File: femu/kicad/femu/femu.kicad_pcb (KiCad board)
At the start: 6 copper layers, 13 x 9.4 mm, 11 parts, among them U1 ESP32-D2WD, U2 FT231XQ, U3 LDO, Y1 ECS-TXO-2016-33-400-TR

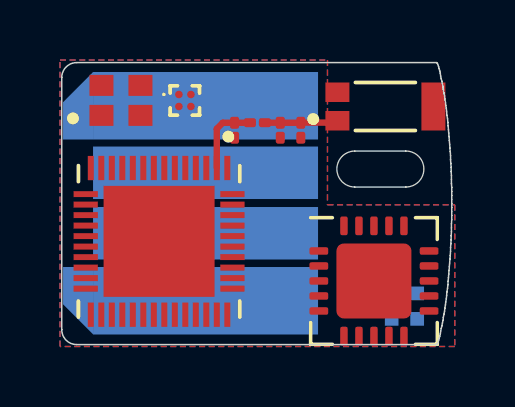
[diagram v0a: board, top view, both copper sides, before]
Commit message: KiCAD design updates
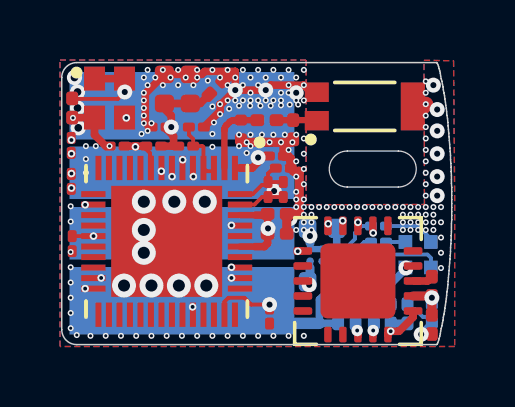
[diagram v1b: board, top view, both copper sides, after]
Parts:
- added C10: 2.2uF, Capacitor_SMD:C_0402_1005Metric, B.Cu at (135.7, 97.7)
- added C11: 2.2uF, Capacitor_SMD:C_0402_1005Metric, B.Cu at (135.7, 99.5)
- added C12: 0.1uF, Capacitor_SMD:C_0201_0603Metric, F.Cu at (127.4, 93.7)
- added C13: 10nF, Capacitor_SMD:C_01005_0402Metric, F.Cu at (134.4, 95.7)
- added C14: 0.22uF, Capacitor_SMD:C_01005_0402Metric, F.Cu at (130.3, 94.4)
- added C15: 2.2uF, Capacitor_SMD:C_0201_0603Metric, F.Cu at (134.2, 97.9)
- added C16: 100pF, Capacitor_SMD:C_0201_0603Metric, F.Cu at (134.2, 97.3)
- added C17: 0.22uF, Capacitor_SMD:C_01005_0402Metric, F.Cu at (127.4, 98.2)
- added C18: 22uF, Capacitor_SMD:C_0402_1005Metric, F.Cu at (130.5, 93.1)
- added C19: 3.3nF, Capacitor_SMD:C_01005_0402Metric, F.Cu at (133.9, 96.4)
- added C20: 270PF, Capacitor_SMD:C_01005_0402Metric, F.Cu at (127.4, 96.2)
- added C21: 0.22uF, Capacitor_SMD:C_01005_0402Metric, F.Cu at (134.0, 100.7)
- added C22: 22uF, Capacitor_SMD:C_0402_1005Metric, F.Cu at (131.3, 93.1)
- added C23: 2.2uF, Capacitor_SMD:C_0201_0603Metric, F.Cu at (132.2, 93.0)
- added C24: 0.22uF, Capacitor_SMD:C_01005_0402Metric, F.Cu at (134.2, 95.3)
- added C25: 0.22uF, Capacitor_SMD:C_01005_0402Metric, F.Cu at (128.9, 95.0)
- added C26: DNP, Capacitor_SMD:C_01005_0402Metric, F.Cu at (131.5, 94.4)
- added C4: 0.22uF, Capacitor_SMD:C_0201_0603Metric, F.Cu at (139.4, 99.7)
- added C5: 4.7uF, Capacitor_SMD:C_0201_0603Metric, F.Cu at (139.4, 100.9)
- added C6: 0.22uF, Capacitor_SMD:C_0201_0603Metric, B.Cu at (138.6, 100.6)
- added C7: 47pF, Capacitor_SMD:C_0201_0603Metric, B.Cu at (137.1, 99.5)
- added C8: 47pF, Capacitor_SMD:C_0201_0603Metric, B.Cu at (136.3, 100.6)
- added C9: 10nF, Capacitor_SMD:C_0201_0603Metric, B.Cu at (139.4, 100.6)
- added L2: L, Inductor_SMD:L_01005_0402Metric, F.Cu at (131.2, 95.0)
- added R1: 0, Resistor_SMD:R_0201_0603Metric, B.Cu at (138.0, 100.6)
- added R2: 27, Resistor_SMD:R_0201_0603Metric, B.Cu at (137.5, 100.6)
- added R3: 27, Resistor_SMD:R_0201_0603Metric, B.Cu at (136.9, 100.6)
- added R4: 270, Resistor_SMD:R_01005_0402Metric, B.Cu at (137.6, 98.2)
- added R5: 270, Resistor_SMD:R_01005_0402Metric, B.Cu at (137.6, 97.7)
- added R6: 270, Resistor_SMD:R_01005_0402Metric, B.Cu at (137.6, 98.8)
- added R7: 10K, Resistor_SMD:R_01005_0402Metric, F.Cu at (130.1, 95.0)
- added R8: 20K (5%), Resistor_SMD:R_01005_0402Metric, F.Cu at (134.4, 96.4)
- C1: value C_Small -> 270PF
- C2, C3: footprint Capacitor_SMD:C_01005_0402Metric -> Capacitor_SMD:C_0201_0603Metric
- L1: footprint Inductor_SMD:L_01005_0402Metric -> Inductor_SMD:L_0201_0603Metric
- U3: moved to B.Cu
- moved C1 7.67 mm to (127.4, 95.0), turned to 90 degrees
- moved U3 6.76 mm to (135.5, 98.6), turned to -90 degrees
- moved LED1 1.77 mm to (138.9, 98.6), turned to -90 degrees
- moved USB1 0.79 mm to (131.1, 96.9)
- moved ANT1 0.69 mm to (137.2, 93.7)
- moved U2 0.53 mm to (136.9, 99.5)
- moved C2 0.43 mm to (134.8, 94.4)
- moved Y1 0.39 mm to (128.7, 93.4), turned to -90 degrees
- moved C3 0.33 mm to (133.9, 94.1)
- moved U1 0.25 mm to (130.6, 98.2)
- moved L1 0.21 mm to (133.0, 94.4)
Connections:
- C1 pad 1: Net-(ANT1-PadFEED) -> Net-(C1-Pad1)
- C1 pad 2: GND -> Net-(C1-Pad2)
- LED1 pad 1: Net-(LED1-Pad1) -> +3V3
- U1 pad 1: Net-(U1-Pad1) -> +3V3
- U1 pad 16: Net-(U1-Pad16) -> /IO27_R
- U1 pad 19: Net-(U1-Pad19) -> +3V3
- U1 pad 23: Net-(U1-Pad23) -> /BOOT_DTR
- U1 pad 24: Net-(U1-Pad24) -> /IO4_G
- U1 pad 34: Net-(U1-Pad34) -> /IO5_B
- U1 pad 37: Net-(U1-Pad37) -> +3V3
- U1 pad 40: Net-(U1-Pad40) -> /UART-
- U1 pad 41: Net-(U1-Pad41) -> /UART+
- U1 pad 43: Net-(U1-Pad1) -> +3V3
- U1 pad 46: Net-(U1-Pad1) -> +3V3
- U1 pad 7: Net-(U1-Pad7) -> Net-(C1-Pad2)
- U1 pad 8: Net-(U1-Pad8) -> Net-(C1-Pad1)
- U1 pad 9: Net-(U1-Pad9) -> /EN_RTS
- U2 pad 1: Net-(U2-Pad1) -> /UART+
- U2 pad 10: Net-(U2-Pad10) -> Net-(C6-Pad1)
- U2 pad 11: Net-(U2-Pad11) -> Net-(C6-Pad1)
- U2 pad 12: Net-(U2-Pad12) -> +5V
- U2 pad 17: Net-(U2-Pad17) -> /UART-
- U2 pad 18: Net-(U2-Pad18) -> /BOOT_DTR
- U2 pad 19: Net-(U2-Pad19) -> /EN_RTS
- U2 pad 20: Net-(U2-Pad20) -> Net-(C6-Pad1)
- U2 pad 8: Net-(U2-Pad8) -> /USB+
- U2 pad 9: Net-(U2-Pad9) -> /USB-
- U3 pad A1: Net-(U3-PadA1) -> +5V
- U3 pad A2: Net-(U3-PadA2) -> +3V3
- U3 pad B1: Net-(U3-PadB1) -> +5V
- USB1 pad 1: Net-(USB1-Pad1) -> GND
- USB1 pad 2: Net-(USB1-Pad2) -> /D+
- USB1 pad 3: Net-(USB1-Pad3) -> /D-
- USB1 pad 4: Net-(USB1-Pad4) -> +5V
- Y1 pad 1: Net-(Y1-Pad1) -> +3V3
- Y1 pad 3: Net-(Y1-Pad3) -> Net-(U1-Pad45)
- Y1 pad 4: Net-(Y1-Pad4) -> +3V3
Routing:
- net +3V3: track 0.00 -> 44.8 mm, vias 0 -> 8
- net GND: track 0.00 -> 36.4 mm, vias 0 -> 197
- net +5V: track 0.00 -> 34.1 mm, vias 0 -> 6
- net /IO27_R: track 0.00 -> 16.8 mm, vias 0 -> 3
- net /D+: track 0.00 -> 12.2 mm, vias 0 -> 2
- net /IO4_G: track 0.00 -> 10.9 mm, vias 0 -> 3
- net /D-: track 0.00 -> 10.8 mm, vias 0 -> 2
- net /EN_RTS: track 0.00 -> 10.4 mm, vias 0 -> 2
- net /BOOT_DTR: track 0.00 -> 9.64 mm, vias 0 -> 2
- net Net-(C6-Pad1): track 0.00 -> 8.96 mm, vias 0 -> 2
- net /IO5_B: track 0.00 -> 8.16 mm, vias 0 -> 3
- net /UART-: track 0.00 -> 7.03 mm, vias 0 -> 2
- net Net-(U1-Pad45): track 0.00 -> 6.62 mm, vias 0 -> 2
- net /UART+: track 0.00 -> 5.28 mm, vias 0 -> 2
- net Net-(C20-Pad1): track 0.00 -> 4.69 mm, vias 0 -> 2
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- added copper zone on In1.Cu, net GND
- removed copper zone on In1.Cu.GND, net (none)
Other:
- outline, holes or cut-outs redrawn
- net class Default removed
